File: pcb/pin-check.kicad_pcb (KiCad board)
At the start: 2 copper layers, 114.5 x 43.1 mm, 39 parts, among them P1 USB_C_Receptacle_USB2.0, SW1 SW_Push, SW2 SW_Push, SW3 SW_Push, SW4 SW_Push, SW5 SW_Push, SW6 SW_Push, SW7 Reset, SW8 Boot, U1 ATmega328P-PU, Y1 16MHz

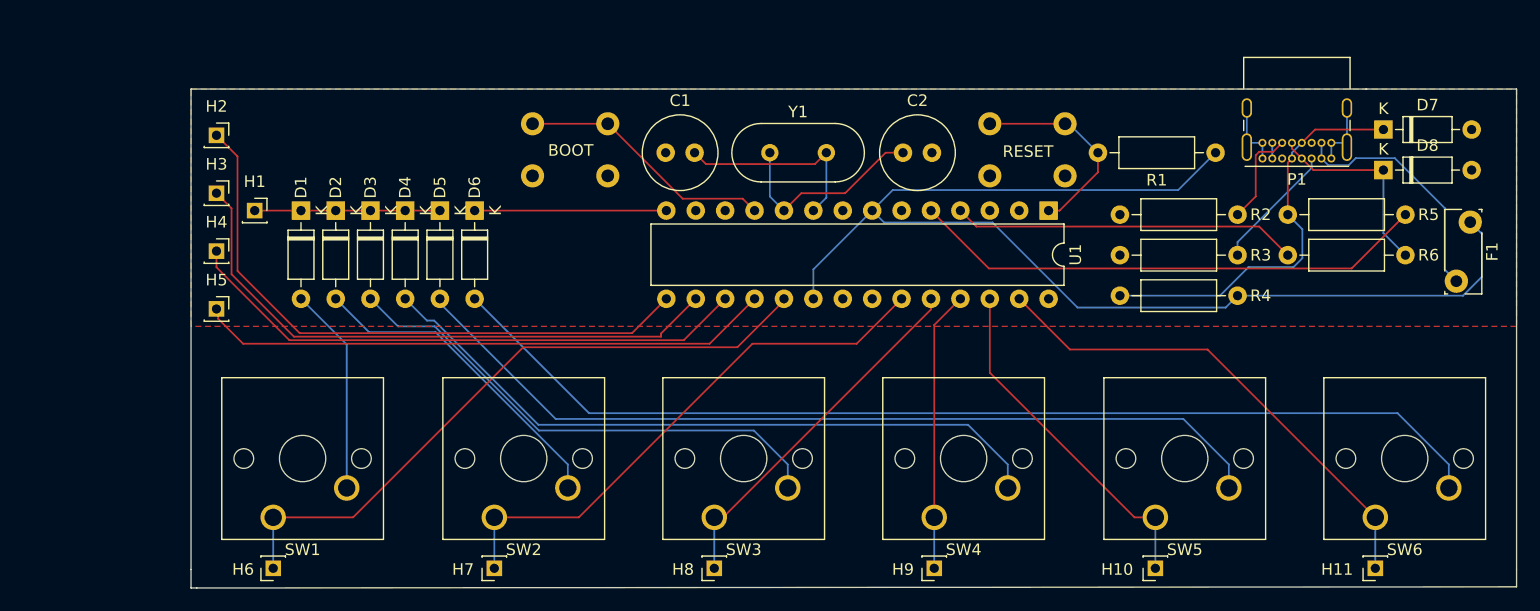
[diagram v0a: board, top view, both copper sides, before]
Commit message: still a wip, uploading bom
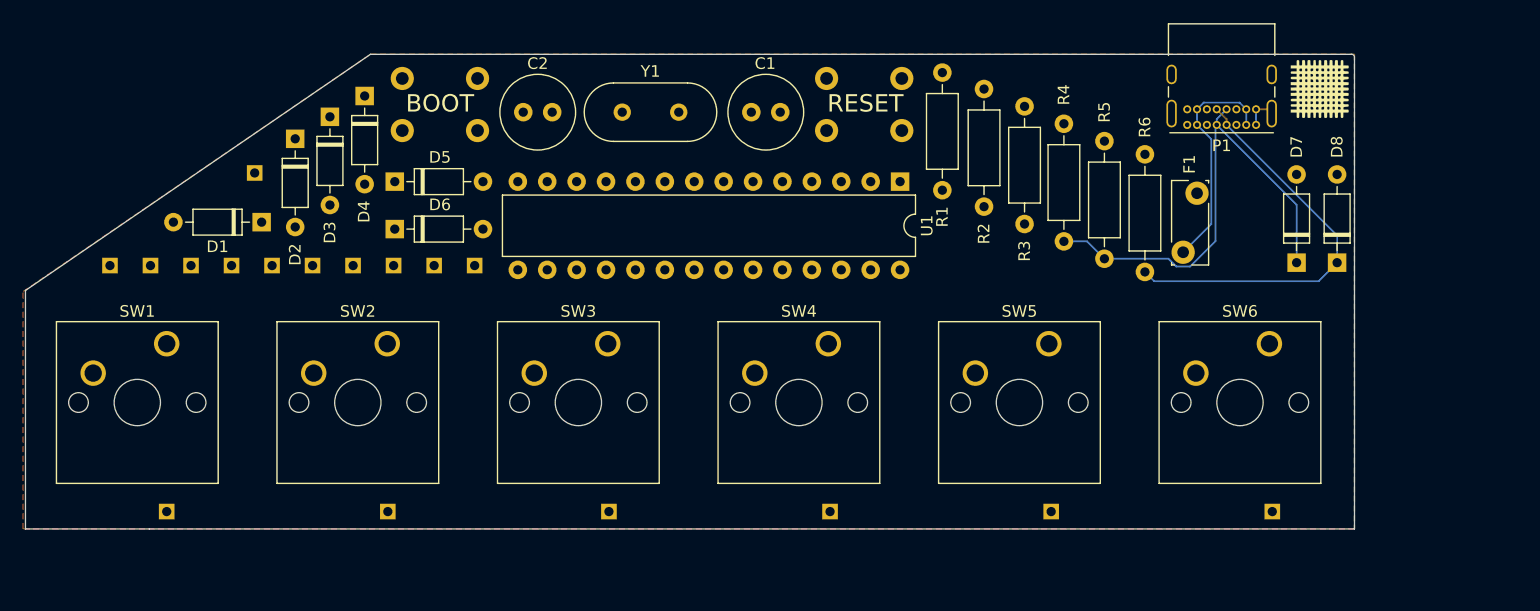
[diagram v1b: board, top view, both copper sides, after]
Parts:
- added G***: LOGO, pin-check:pin-check, F.Cu at (265.0, 70.0)
- added H12: Pad, Connector_PinSocket_2.00mm:PinSocket_1x01_P2.00mm_Vertical, B.Cu at (178.0, 85.2)
- added H13: Pad, Connector_PinSocket_2.00mm:PinSocket_1x01_P2.00mm_Vertical, B.Cu at (174.5, 85.2)
- added H14: Pad, Connector_PinSocket_2.00mm:PinSocket_1x01_P2.00mm_Vertical, B.Cu at (171.0, 85.2)
- added H15: Pad, Connector_PinSocket_2.00mm:PinSocket_1x01_P2.00mm_Vertical, B.Cu at (167.5, 85.2)
- added H16: Pad, Connector_PinSocket_2.00mm:PinSocket_1x01_P2.00mm_Vertical, B.Cu at (164.0, 85.2)
- added H17: Pad, Connector_PinSocket_2.00mm:PinSocket_1x01_P2.00mm_Vertical, B.Cu at (160.5, 85.2)
- H1, H10, H11, H2, H3, H4, H5, H6, H7, H8, H9: moved to B.Cu
- moved H11 92.1 mm to (181.5, 85.2)
- moved H10 70.8 mm to (185.0, 85.2)
- moved H6 67.4 mm to (241.8, 106.5)
- moved H7 67.4 mm to (260.9, 106.5)
- moved H5 55.8 mm to (222.7, 106.5), turned to 180 degrees
- moved H9 50.5 mm to (188.5, 85.2)
- moved H4 40.7 mm to (203.6, 106.5), turned to 180 degrees
- moved C2 35.5 mm to (196.2, 72.0), turned to 0 degrees
- moved H8 33.4 mm to (192.0, 85.2)
- moved H2 32.8 mm to (165.4, 106.5), turned to 180 degrees
- moved H3 31.2 mm to (184.5, 106.5), turned to 180 degrees
- moved R5 26.8 mm to (246.4, 74.5), turned to 270 degrees
- moved R2 24.4 mm to (236.0, 70.0), turned to 270 degrees
- moved R1 23.8 mm to (232.4, 78.7), turned to 90 degrees
- moved F1 23.7 mm to (254.4, 79.0)
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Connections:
- H10 pad 1: /Col4 -> /B3
- H11 pad 1: /Col5 -> /B4
- H2 pad 1: /Row1 -> /Col0
- H3 pad 1: /Row2 -> /Col1
- H4 pad 1: /Row3 -> /Col2
- H5 pad 1: /Row4 -> /Col3
- H6 pad 1: /Col0 -> /Col4
- H7 pad 1: /Col1 -> /Col5
- H8 pad 1: /Col2 -> /B1
- H9 pad 1: /Col3 -> /B2
- U1 pad 12: Net-(U1-Pad12) -> /D6
- U1 pad 13: Net-(U1-Pad13) -> /D7
- U1 pad 15: /Row1 -> /B1
- U1 pad 16: /Row2 -> /B2
- U1 pad 17: /Row3 -> /B3
- U1 pad 18: /Row4 -> /B4
- U1 pad 2: Net-(U1-Pad2) -> /D0
- U1 pad 28: Net-(U1-Pad28) -> /C5
- U1 pad 3: Net-(U1-Pad3) -> /D1
- U1 pad 6: Net-(U1-Pad6) -> /D4
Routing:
- net +5V: track 103.8 -> 0.00 mm
- net Net-(D6-Pad2): track 92.7 -> 0.00 mm
- net Net-(D5-Pad2): track 76.7 -> 0.00 mm
- net Net-(D4-Pad2): track 60.4 -> 0.00 mm
- net /Col0: track 56.4 -> 0.00 mm
- net /Row1: track 53.0 -> 0.00 mm
- net /Row2: track 51.4 -> 0.00 mm
- net /Row4: track 49.7 -> 0.00 mm
- net /Row3: track 49.4 -> 0.00 mm
- net /Col1: track 47.4 -> 0.00 mm
- net /D-: track 45.0 -> 0.00 mm
- net Net-(D3-Pad2): track 44.0 -> 0.00 mm
- net /Col5: track 43.7 -> 0.00 mm
- net /Row0: track 32.6 -> 0.00 mm
- net /Col2: track 31.5 -> 0.00 mm
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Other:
- board size 114.5 x 43.1 mm -> 114.8 x 41 mm

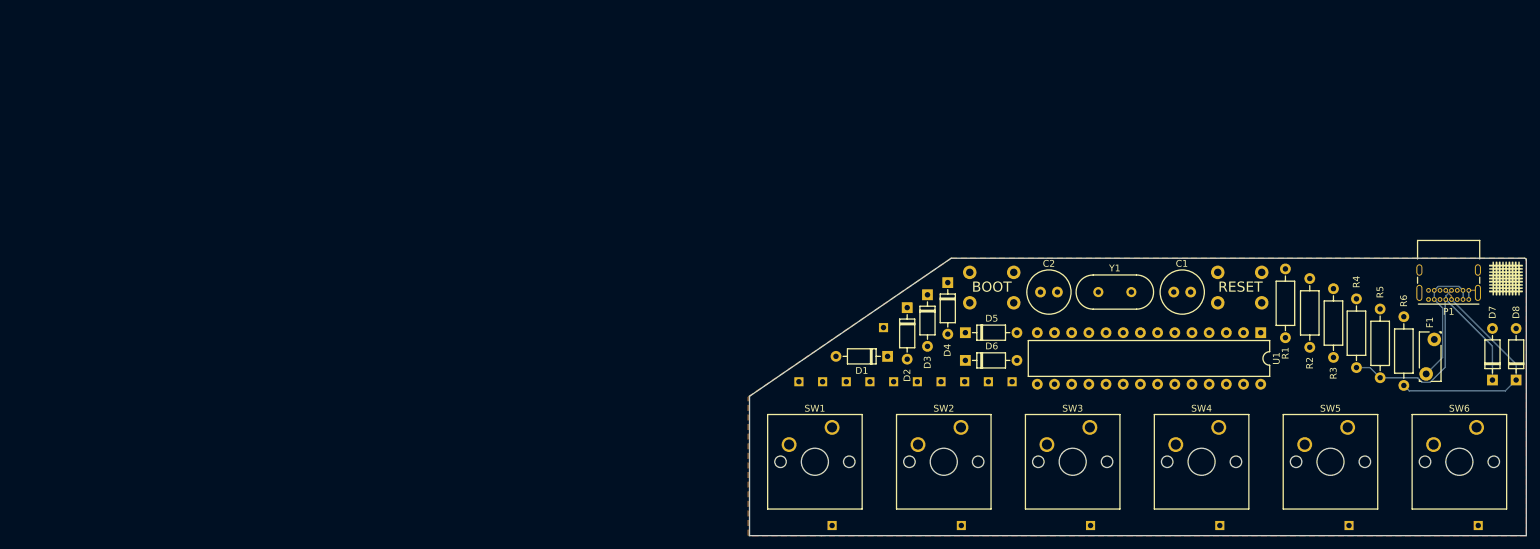
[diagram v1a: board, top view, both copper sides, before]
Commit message: a bunch of changes, update bom, new render
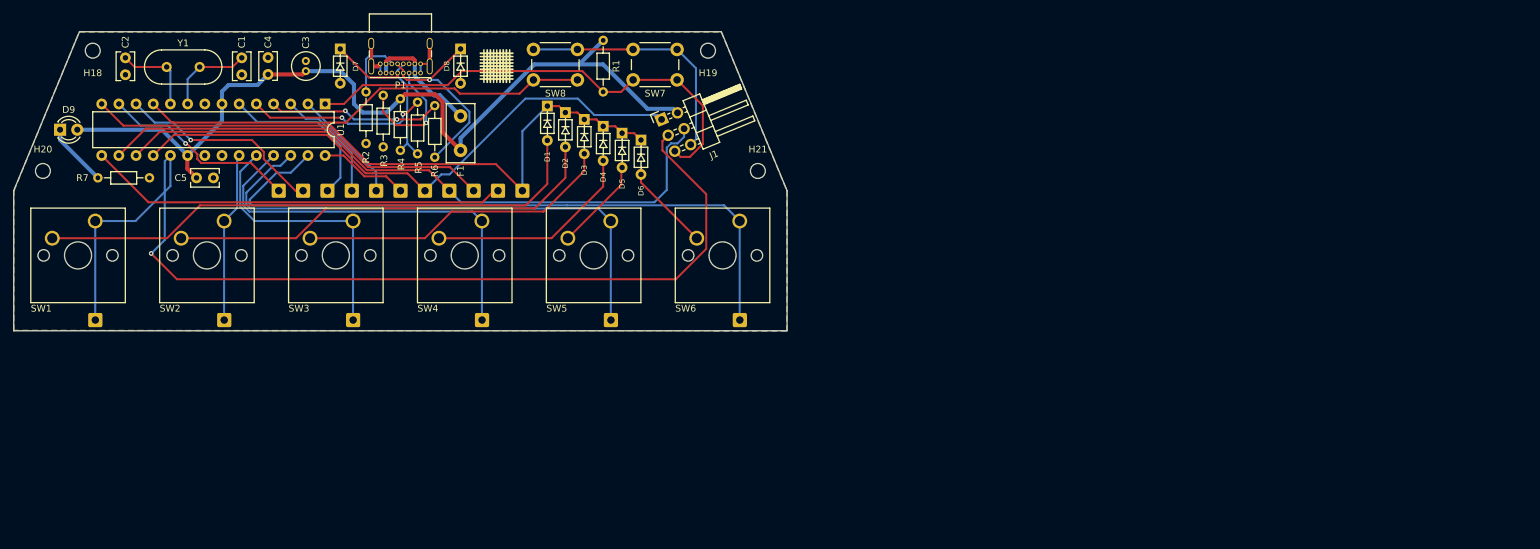
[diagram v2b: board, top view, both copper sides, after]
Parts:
- added C3: 4.7u, Capacitor_THT:C_Radial_D4.0mm_H7.0mm_P1.50mm, F.Cu at (87.6, 37.8)
- added C4: 0.1u, Capacitor_THT:C_Rect_L4.0mm_W2.5mm_P2.50mm, F.Cu at (82.0, 37.3)
- added C5: 0.1u, Capacitor_THT:C_Rect_L4.0mm_W2.5mm_P2.50mm, F.Cu at (74.0, 55.1)
- added D9: LED, LED_THT:LED_D3.0mm, F.Cu at (51.3, 48.0)
- added H18: MountingHole, MountingHole:MountingHole_2.2mm_M2, F.Cu at (56.1, 36.3)
- added H19: MountingHole, MountingHole:MountingHole_2.2mm_M2, F.Cu at (147.1, 36.3)
- added H20: MountingHole, MountingHole:MountingHole_2.2mm_M2, F.Cu at (48.8, 54.1)
- added H21: MountingHole, MountingHole:MountingHole_2.2mm_M2, F.Cu at (154.4, 54.1)
- added J1: AVR-ISP-6, Connector_PinHeader_2.54mm:PinHeader_2x03_P2.54mm_Horizontal, F.Cu at (140.2, 46.5)
- added R7: 1.5k, Resistor_THT:R_Axial_DIN0204_L3.6mm_D1.6mm_P7.62mm_Horizontal, F.Cu at (56.9, 55.1)
- C1, C2: footprint Capacitor_THT:C_Radial_D6.3mm_H5.0mm_P2.50mm -> Capacitor_THT:C_Rect_L4.0mm_W2.5mm_P2.50mm
- D1, D2, D3, D4, D5, D6, D7, D8: footprint Diode_THT:D_DO-35_SOD27_P7.62mm_Horizontal -> pin-check:D_DO-35_SOD27_P5.08mm_Horizontal
- F1: footprint Fuse:Fuse_Bourns_MF-RG300 -> Fuse:Fuse_Littelfuse_395Series
- H1, H10, H11, H12, H13, H14, H15, H16, H17, H2, H3, H4, H5, H6, H7, H8, H9: footprint Connector_PinSocket_2.00mm:PinSocket_1x01_P2.00mm_Vertical -> Connector_Wire:SolderWire-0.5sqmm_1x01_D0.9mm_OD2.1mm
- R1, R2, R3, R4, R5, R6: footprint Resistor_THT:R_Axial_DIN0207_L6.3mm_D2.5mm_P10.16mm_Horizontal -> Resistor_THT:R_Axial_DIN0204_L3.6mm_D1.6mm_P7.62mm_Horizontal
- SW7, SW8: moved to F.Cu
- moved D7 177.5 mm to (92.7, 34.8), turned to 270 degrees
- moved D8 163.9 mm to (110.5, 34.8), turned to 270 degrees
- moved P1 158.5 mm to (104.6, 39.6)
- moved G*** 152.4 mm to (115.8, 38.6)
- moved R6 147.1 mm to (106.7, 52.1)
- moved F1 146.6 mm to (110.5, 51.1), turned to 90 degrees
- moved R5 145.5 mm to (104.1, 43.9)
- moved R4 144.4 mm to (101.6, 43.4)
- moved C1 143.9 mm to (78.2, 39.9), turned to 90 degrees
- moved R3 143.3 mm to (99.1, 42.9)
- moved U1 142.3 mm to (90.5, 44.2)
- moved R2 142.2 mm to (96.5, 42.4)
- moved Y1 141.7 mm to (67.1, 38.7)
- moved C2 139.0 mm to (61.0, 39.9), turned to 90 degrees
- moved H7 113.3 mm to (151.8, 76.1)
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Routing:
- net /Col0: track 0.00 -> 153.4 mm, vias 0 -> 1
- net +5V: track 0.00 -> 127.6 mm
- net /Col5: track 0.00 -> 100.1 mm
- net /Row0: track 0.00 -> 97.4 mm
- net /B3: track 0.00 -> 95.6 mm
- net /B4: track 0.00 -> 86.7 mm
- net Net-(D1-Pad2): track 0.00 -> 82.9 mm
- net /Col4: track 0.00 -> 80.1 mm
- net /Reset: track 0.00 -> 72.4 mm
- net /Boot: track 0.00 -> 67.1 mm
- net Net-(D2-Pad2): track 0.00 -> 65.1 mm
- net /B1: track 0.00 -> 62.1 mm
- net /Col3: track 0.00 -> 60.1 mm
- net /B2: track 0.00 -> 58.4 mm
- net Net-(D3-Pad2): track 0.00 -> 47.2 mm
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- added copper zone on B.Cu, net (none)
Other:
- board size 114.8 x 41 mm -> 114.3 x 44.2 mm
- board text removed: "BOOT"
- board text removed: "RESET"
